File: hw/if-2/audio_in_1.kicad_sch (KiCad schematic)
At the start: 0 parts

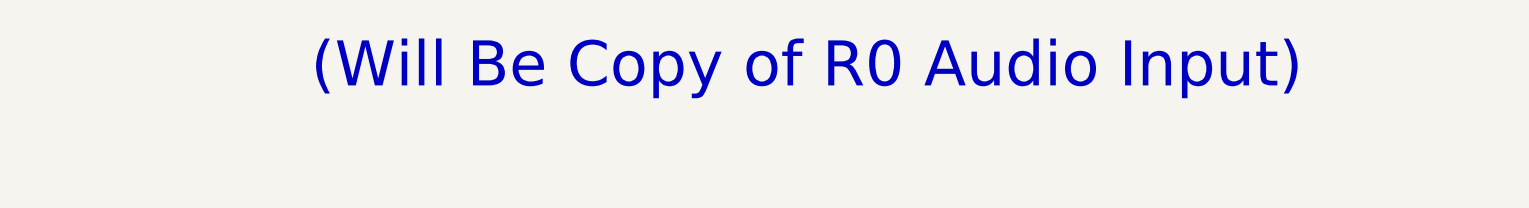
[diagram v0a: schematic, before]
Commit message: First draft of schematic
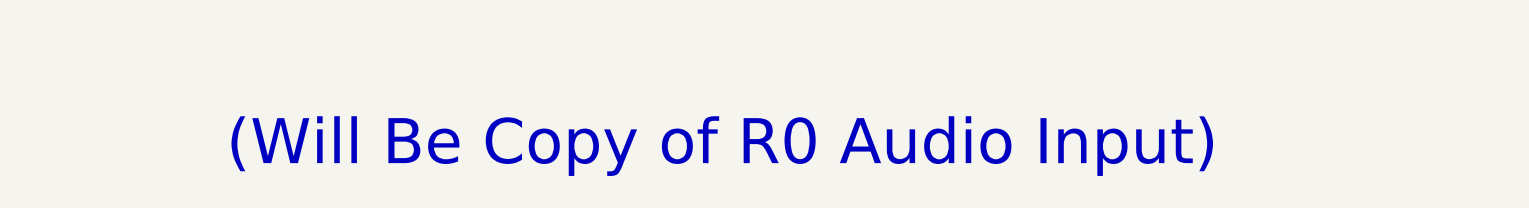
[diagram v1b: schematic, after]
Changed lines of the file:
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@@
 	(text "(Will Be Copy of R0 Audio Input)"
 		(exclude_from_sim no)
-		(at 149.86 92.964 0)
+		(at 140.462 101.6 0)
 		(effects
 			(font
